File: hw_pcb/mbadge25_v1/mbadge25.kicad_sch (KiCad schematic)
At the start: 25 parts, among them J1 USB4105-GF-A, J2 BAT, J3 OLED_I2C, T1 LP0404N3T5G, U1 ESP32-C3-MINI-1, U2 XC6220B331MR

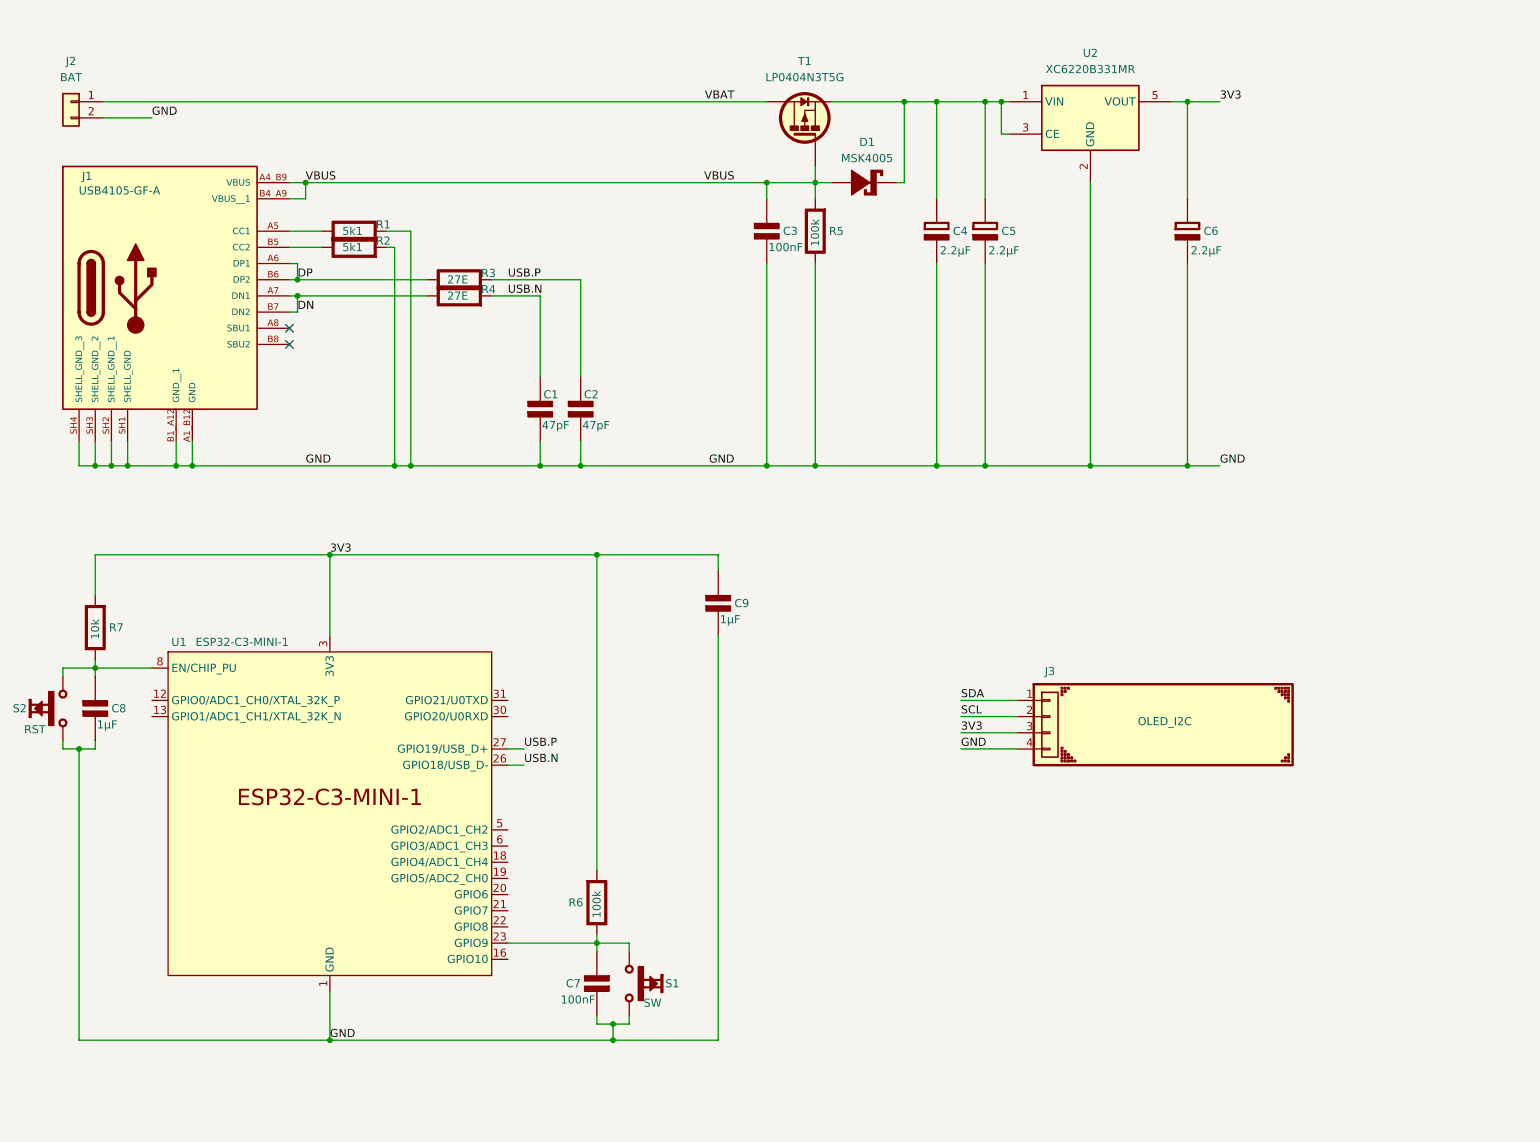
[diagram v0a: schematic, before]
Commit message: v1 draft PCB layout
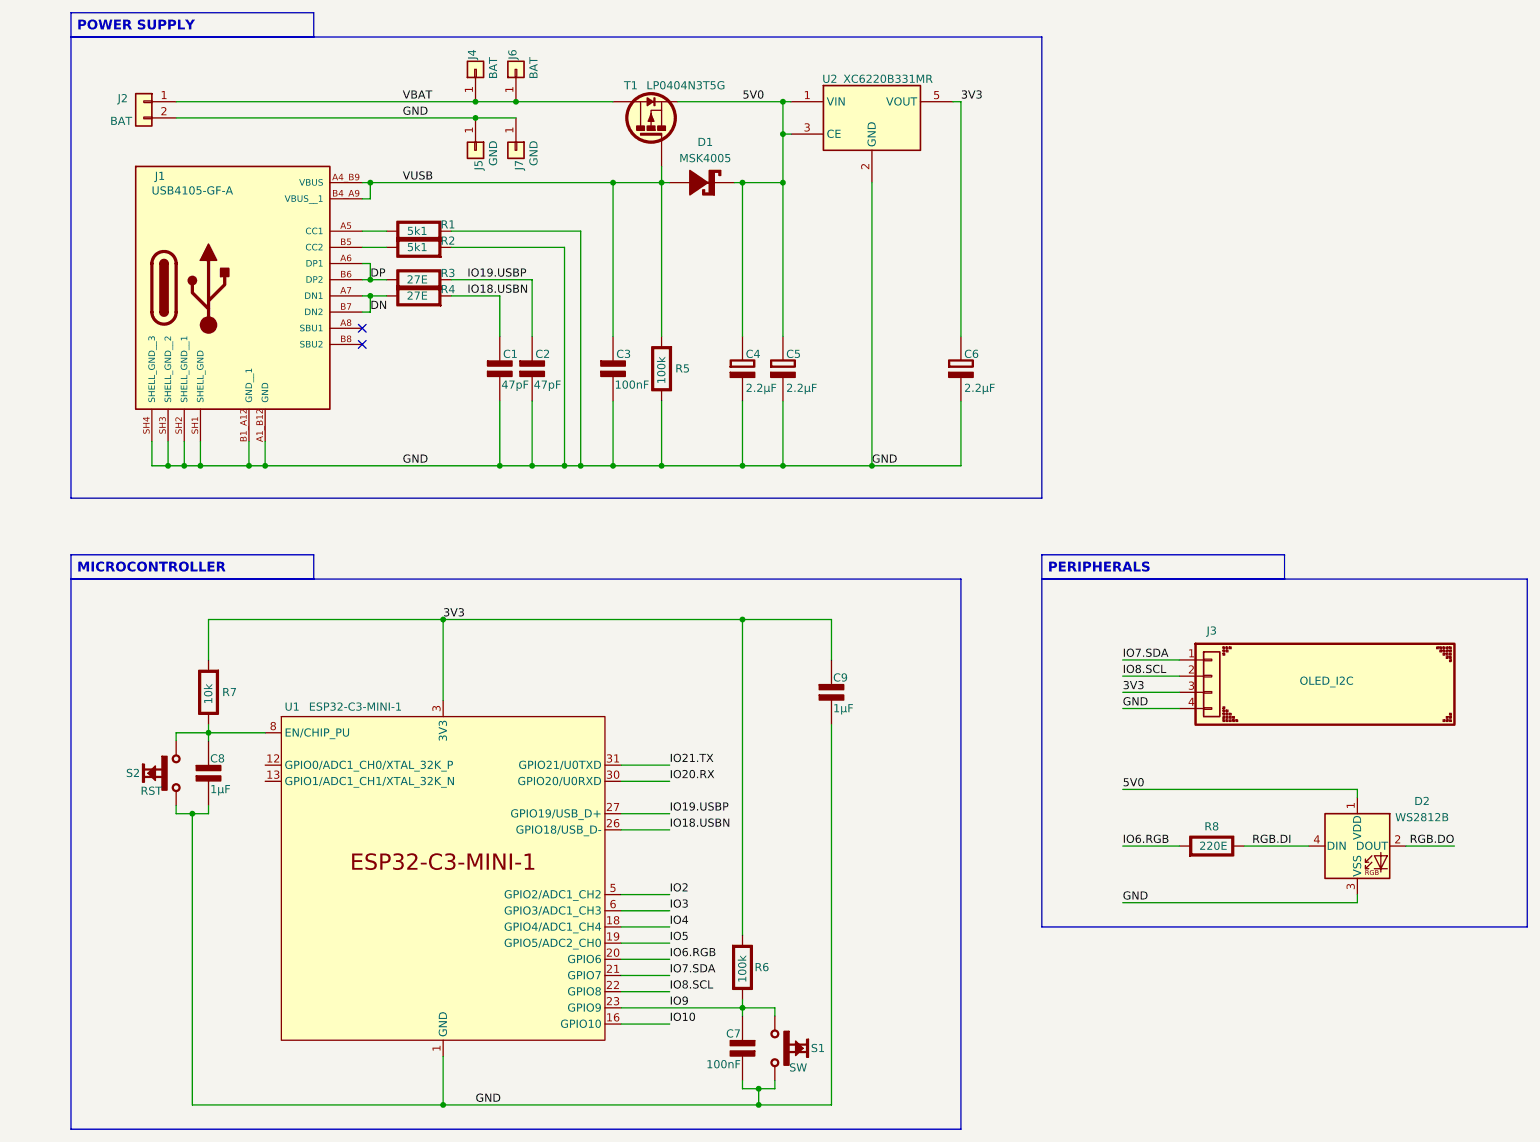
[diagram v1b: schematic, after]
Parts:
- added D2: WS2812B, Library_FP_mbadge25:LED_WS2812B_PLCC4_5.0x5.0mm_P3.2mm, symbol Library_SYM_mbadge25:WS2812B
- added J4: BAT, Library_FP_mbadge25:Pad_6.0mm_Drill3.0mm, symbol Library_SYM_mbadge25:Conn_01x01
- added J5: GND, Library_FP_mbadge25:Pad_6.0mm_Drill3.0mm, symbol Library_SYM_mbadge25:Conn_01x01
- added J6: BAT, Library_FP_mbadge25:Pad_1.2mm_Drill0.7mm, symbol Library_SYM_mbadge25:Conn_01x01
- added J7: GND, Library_FP_mbadge25:Pad_1.2mm_Drill0.7mm, symbol Library_SYM_mbadge25:Conn_01x01
- added R8: 220E, Library_FP_mbadge25:R_1206_3216Metric_Pad1.30x1.75mm, symbol Library_SYM_mbadge25:R
- C1, C2, C3, C7, C8, C9: footprint PCM_Capacitor_SMD_AKL:C_0805_2012Metric_Pad1.18x1.45mm_HandSolder -> Library_FP_mbadge25:C_1206_3216Metric_Pad1.33x1.80mm
- C4, C5, C6: footprint PCM_Capacitor_SMD_AKL:CP_Elec_6.3x5.9 -> Library_FP_mbadge25:C_1206_3216Metric_Pad1.33x1.80mm
- D1: footprint (none) -> Library_FP_mbadge25:D_SOD-523
- J2: footprint (none) -> Library_FP_mbadge25:PinHeader_1x02_P2.54mm_Vertical
- J3: footprint (none) -> Library_FP_mbadge25:OLED_128x32
- R1, R2, R3, R4, R5, R6, R7: footprint Resistor_SMD:R_0805_2012Metric -> Library_FP_mbadge25:R_1206_3216Metric_Pad1.30x1.75mm
- S1, S2: footprint Button_Switch_THT:SW_PUSH_6mm -> Library_FP_mbadge25:SW_SPST
- T1: footprint (none) -> Library_FP_mbadge25:SOT-23-3
- U1: footprint PCM_Espressif:ESP32-C3-MINI-1 -> Library_FP_mbadge25:ESP32-C3-MINI-1
- U2: footprint Package_TO_SOT_SMD:SOT-23-5 -> Library_FP_mbadge25:SOT-23-5_HandSoldering
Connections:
- net SCL is gone; now on net IO8.SCL: J3.2 (Pin_2)
- net SDA is gone; now on net IO7.SDA: J3.1 (Pin_1)
- net GND: now also S1.2, S2.2, D2.3 (VSS), J5.1 (Pin_1), J7.1 (Pin_1); no longer S1.3, S2.3
- net VBAT: now also J4.1 (Pin_1), J6.1 (Pin_1)
- net at C8.1 (+), R7.1 (+), U1.8 (EN/CHIP_PU): now also S2.1; no longer S2.4
- net 5V0: now reaches C4.1 (+), C5.1 (+), D1.1 (K-), T1.3 (S), U2.1 (VIN), U2.3 (CE)
- net 5V0: now also D2.1 (VDD)
- net IO9: now reaches C7.1 (+), R6.1 (+), U1.23 (GPIO9)
- net IO9: now also S1.1; no longer S1.4
- net IO10: now reaches U1.16 (GPIO10)
- net IO4: now reaches U1.18 (GPIO4/ADC1_CH4)
- net IO5: now reaches U1.19 (GPIO5/ADC2_CH0)
- net IO6.RGB: now reaches U1.20 (GPIO6)
- net IO6.RGB: now also R8.2 (-)
- net IO7.SDA: now reaches U1.21 (GPIO7)
- net IO8.SCL: now reaches U1.22 (GPIO8)
- net IO20.RX: now reaches U1.30 (GPIO20/U0RXD)
- net IO21.TX: now reaches U1.31 (GPIO21/U0TXD)
- net IO2: now reaches U1.5 (GPIO2/ADC1_CH2)
- net IO3: now reaches U1.6 (GPIO3/ADC1_CH3)
- net USB.N renamed IO18.USBN
- net USB.P renamed IO19.USBP
- net VBUS renamed VUSB
- new net RGB.DI: D2.4 (DIN), R8.1 (+)
- new net RGB.DO: D2.2 (DOUT)
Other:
- moved on the sheet: C1, C2, C3, C4, C5, C6, C7, C8, C9, D1, J1, J2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
